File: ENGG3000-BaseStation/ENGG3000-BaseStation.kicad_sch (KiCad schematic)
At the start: 57 parts, among them J1 OLED, J10 Cell/Pack 1, J2 Buttons, J3 UltrasonicA, J4 UltrasonicB, J5 USB_C_Receptacle_USB2.0_16P, J7 Power Switch, J8 Cell 3, J9 Cell 2, Q1 SS8050, Q2 AO3401A, SW1 RESET, SW2 BOOT, U1 ESP32-S3-WROOM-1-N16R8, U2 TPS63001DRCR, U3 CN3085

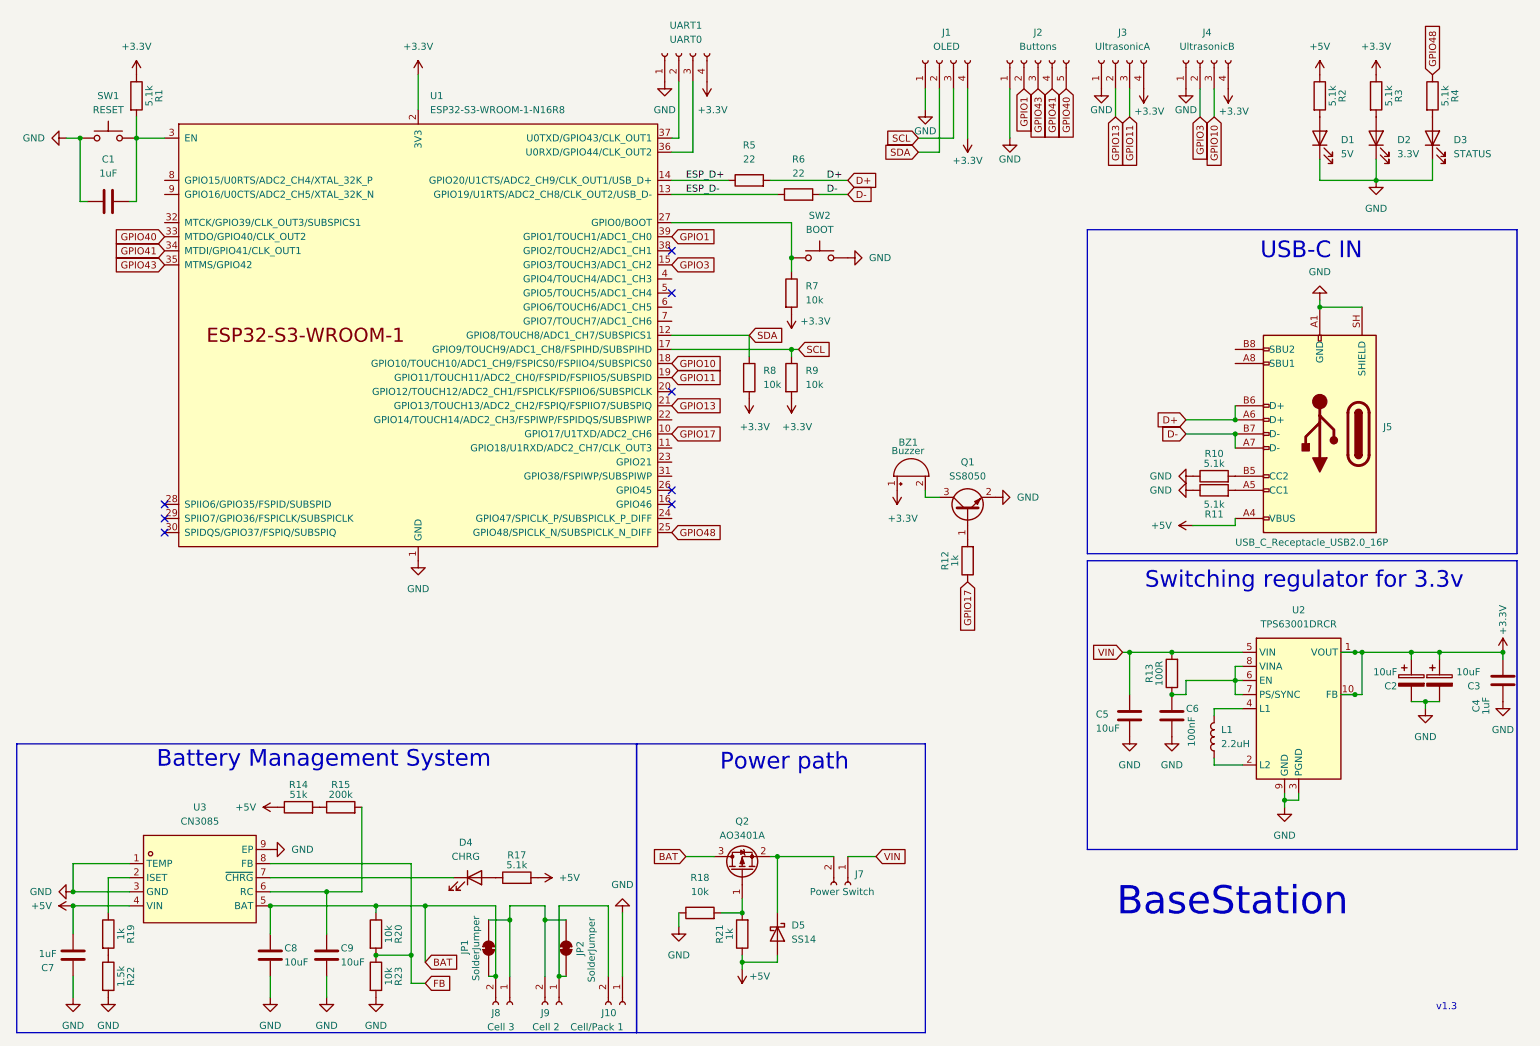
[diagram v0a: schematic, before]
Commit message: Production ready PCB
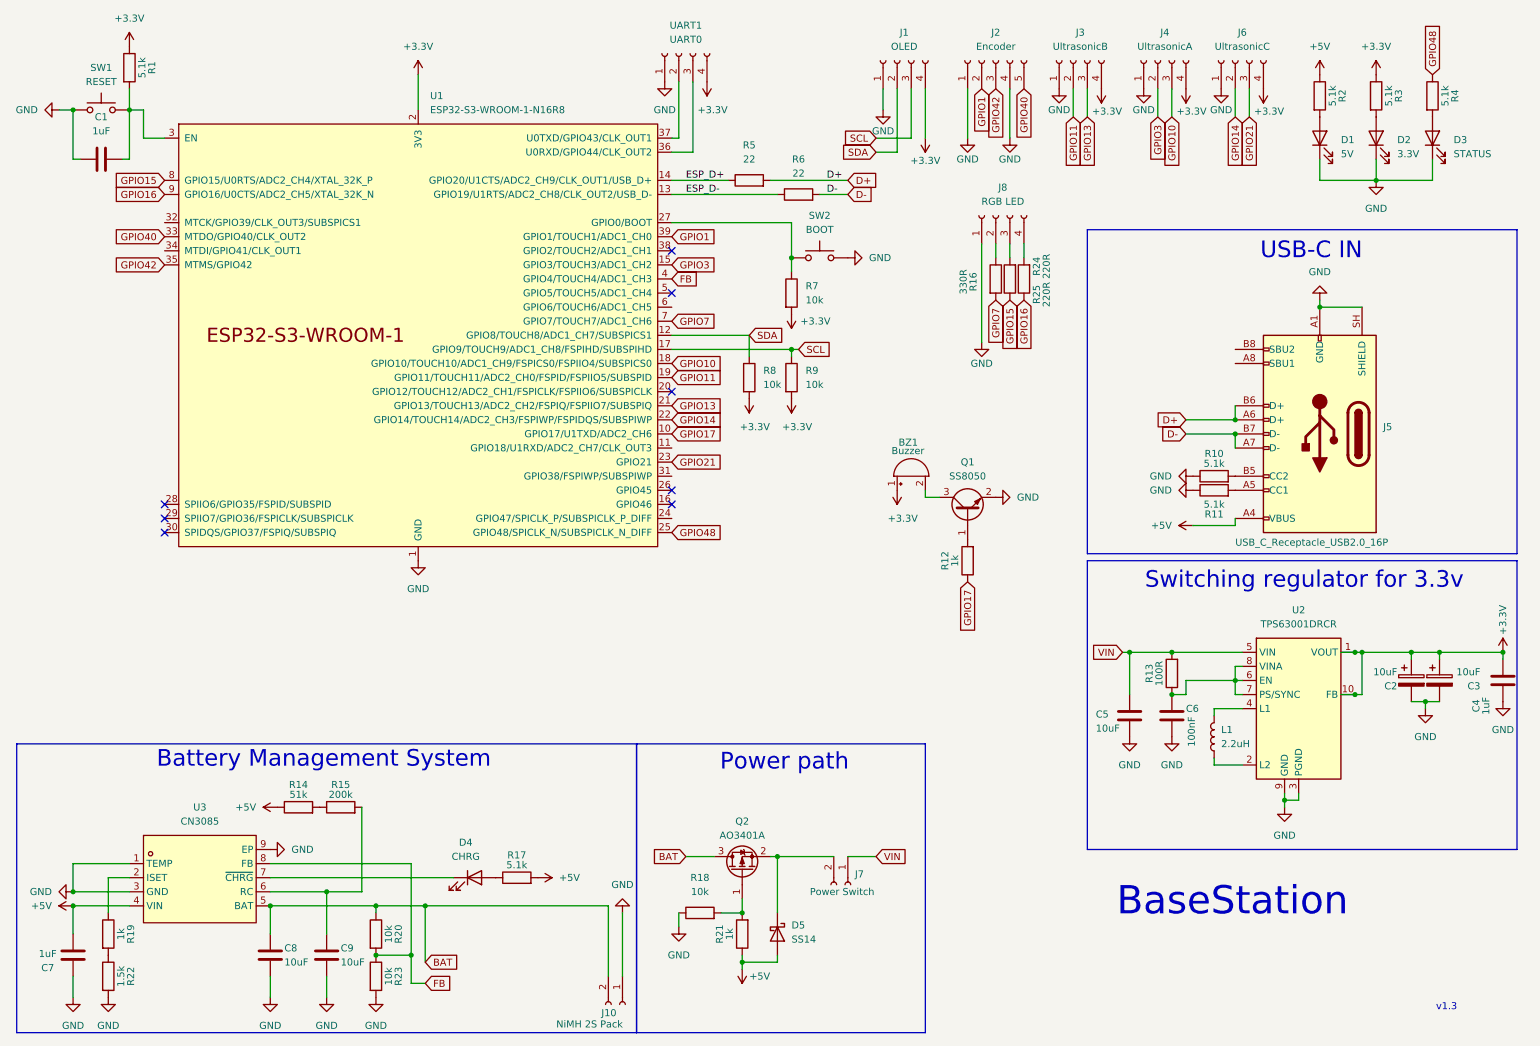
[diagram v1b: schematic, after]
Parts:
- removed J8: Cell 3, Connector_JST:JST_XH_B2B-XH-A_1x02_P2.50mm_Vertical, symbol Connector:Conn_01x02_Socket
- removed J9: Cell 2, Connector_JST:JST_XH_B2B-XH-A_1x02_P2.50mm_Vertical, symbol Connector:Conn_01x02_Socket
- removed JP1, JP2: SolderJumper, Jumper:SolderJumper-2_P1.3mm_Bridged2Bar_RoundedPad1.0x1.5mm, symbol Jumper:SolderJumper_2_Bridged
- added J6: UltrasonicC, Connector_PinHeader_2.54mm:PinHeader_1x04_P2.54mm_Vertical, symbol Connector:Conn_01x04_Socket
- added J8: RGB LED, Connector_PinHeader_2.54mm:PinHeader_1x04_P2.54mm_Vertical, symbol Connector:Conn_01x04_Socket
- added R16: 330R, Resistor_SMD:R_0402_1005Metric, symbol Device:R
- added R24, R25: 220R, Resistor_SMD:R_0402_1005Metric, symbol Device:R
- J10: value Cell/Pack 1 -> NiMH 2S Pack
- J2: value Buttons -> Encoder
- J3: value UltrasonicA -> UltrasonicB
- J4: value UltrasonicB -> UltrasonicA
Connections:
- net +3.3V: now also J6.4 (3.3V)
- net BAT: now also J10.2 (+)
- net FB: now also U1.4 (GPIO4/TOUCH4/ADC1_CH3)
- net GND: now also J2.4 (Button_C), J6.1 (GND), J8.1 (GND)
- net GPIO11: now also J3.2 (TRIG); no longer J3.3 (ECHO)
- net GPIO13: now also J3.3 (ECHO); no longer J3.2 (TRIG)
- net GPIO14: now reaches U1.22 (GPIO14/TOUCH14/ADC2_CH3/FSPIWP/FSPIDQS/SUBSPIWP)
- net GPIO14: now also J6.2 (TRIG)
- net GPIO21: now reaches U1.23 (GPIO21)
- net GPIO21: now also J6.3 (ECHO)
- net GPIO7: now reaches U1.7 (GPIO7/TOUCH7/ADC1_CH6)
- net GPIO7: now also R16.2
- net GPIO15: now reaches U1.8 (GPIO15/U0RTS/ADC2_CH4/XTAL_32K_P)
- net GPIO15: now also R24.1
- net GPIO16: now reaches U1.9 (GPIO16/U0CTS/ADC2_CH5/XTAL_32K_N)
- net GPIO16: now also R25.1
- net GPIO41: no longer names the net of U1.34 (MTDI/GPIO41/CLK_OUT1)
- net GPIO41: no longer J2.4 (Button_C)
- net GPIO43 renamed GPIO42
- new net: J8.2 (R), R16.1
- new net: J8.3 (G), R24.2
- new net: J8.4 (B), R25.2
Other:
- moved on the sheet: C1, J1, J2, J3, J4, R1, SW1
